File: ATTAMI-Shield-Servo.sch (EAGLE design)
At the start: 12 parts

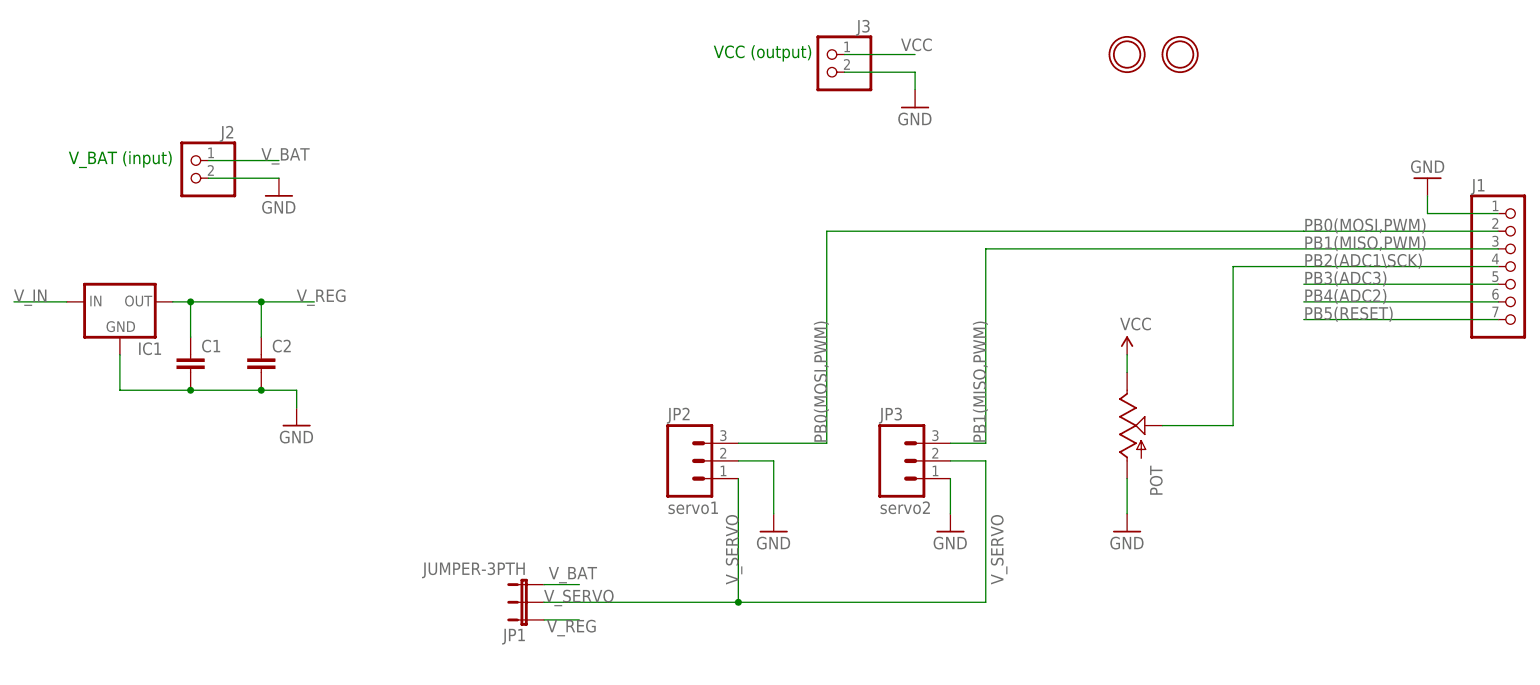
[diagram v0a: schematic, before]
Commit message: servo shield
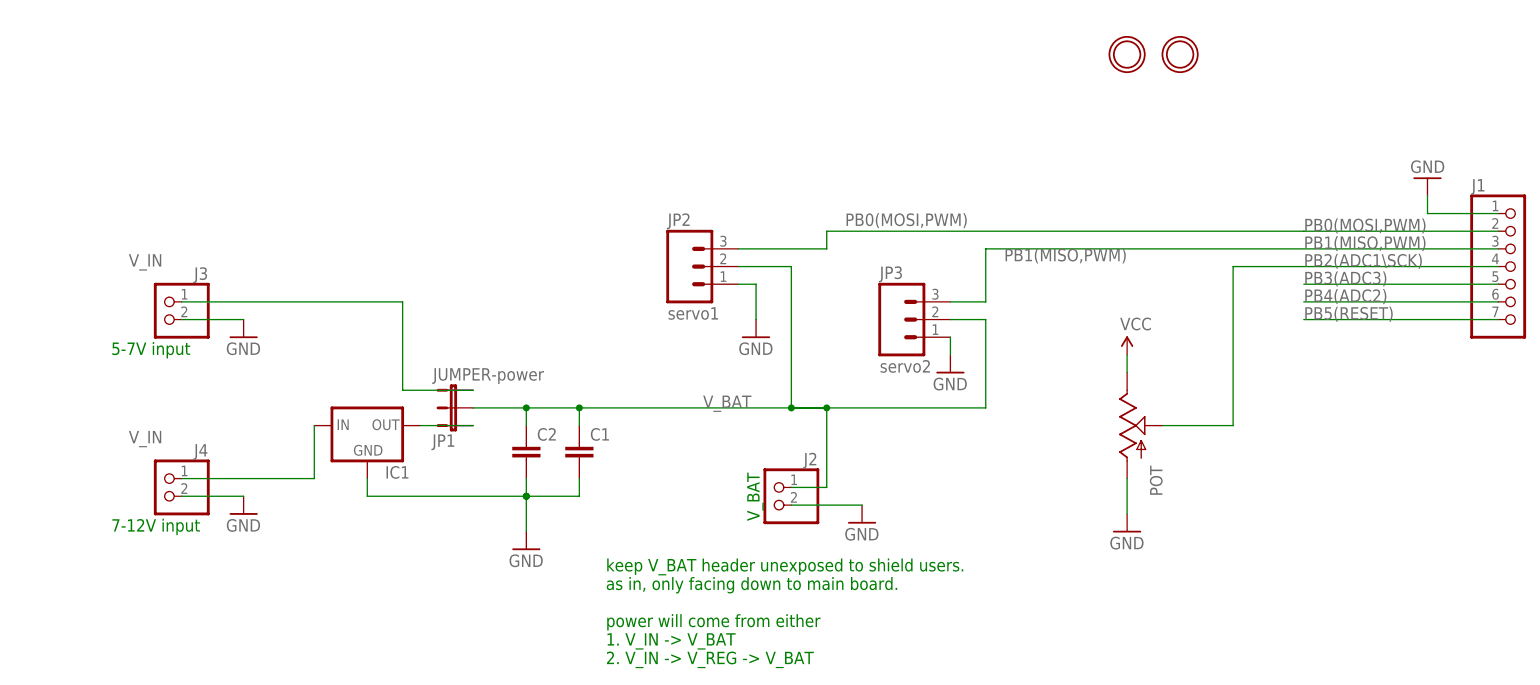
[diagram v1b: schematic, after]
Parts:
- added J4: (no value), microbuilder:HEADER-1X2ROUND
- JP1: value JUMPER-3PTH -> JUMPER-power
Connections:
- removed net V_REG: C1.1, C2.1, IC1.OUT, JP1.1
- removed net V_SERVO: JP1.2, JP3.2
- new net N$3: IC1.OUT, JP1.1
- net GND: now also J4.2, JP2.1, JP3.1; no longer JP2.2
- net VCC: no longer J3.1
- net V_BAT: now also C1.1, C2.1, JP1.2, JP2.2, JP3.2; no longer JP1.3
- net V_IN: now also J3.1, J4.1, JP1.3
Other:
- note added: "5-7V input"
- note added: "7-12V input"
- note added: "V_BAT"
- note added: "keep V_BAT header unexposed to shield users. as in, only facing down to main board. power will come from either 1. V_IN -> V_BAT 2. V_IN -> V_REG -> V_BAT"
- note added: "more at github.com/telavivmakers/at-tami Notes:"
- note removed: "VCC (output)"
- note removed: "V_BAT (input)"
- note removed: "more at github.com/telavivmakers/at-tami Notes: 1. D1 and D2 are Blue LEDs they might not light when using Vi_BAT <4V~ 2. When VCC is less than 5V change the system clock of the ATTINY85 to 8MHz or less - refer to the datasheet P163 Section 21-3 Speed"
- moved on the sheet: C1, C2, IC1, J2, J3, JP1, JP2, JP3
